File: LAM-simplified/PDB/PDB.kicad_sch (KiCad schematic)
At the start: 22 parts, among them J1 Conn_02x03_Counter_Clockwise, J10 Conn_01x02, J11 Conn_01x02, J12 Conn_01x02, J13 Conn_01x02, J14 Conn_01x02, J15 Conn_01x02, J16 Conn_01x02, J2 Conn_02x03_Counter_Clockwise, J3 Conn_02x03_Counter_Clockwise, J4 Conn_02x03_Counter_Clockwise, J5 Conn_01x02, J6 Conn_01x02, J7 Conn_01x02, J8 Conn_01x02, J9 Conn_01x02

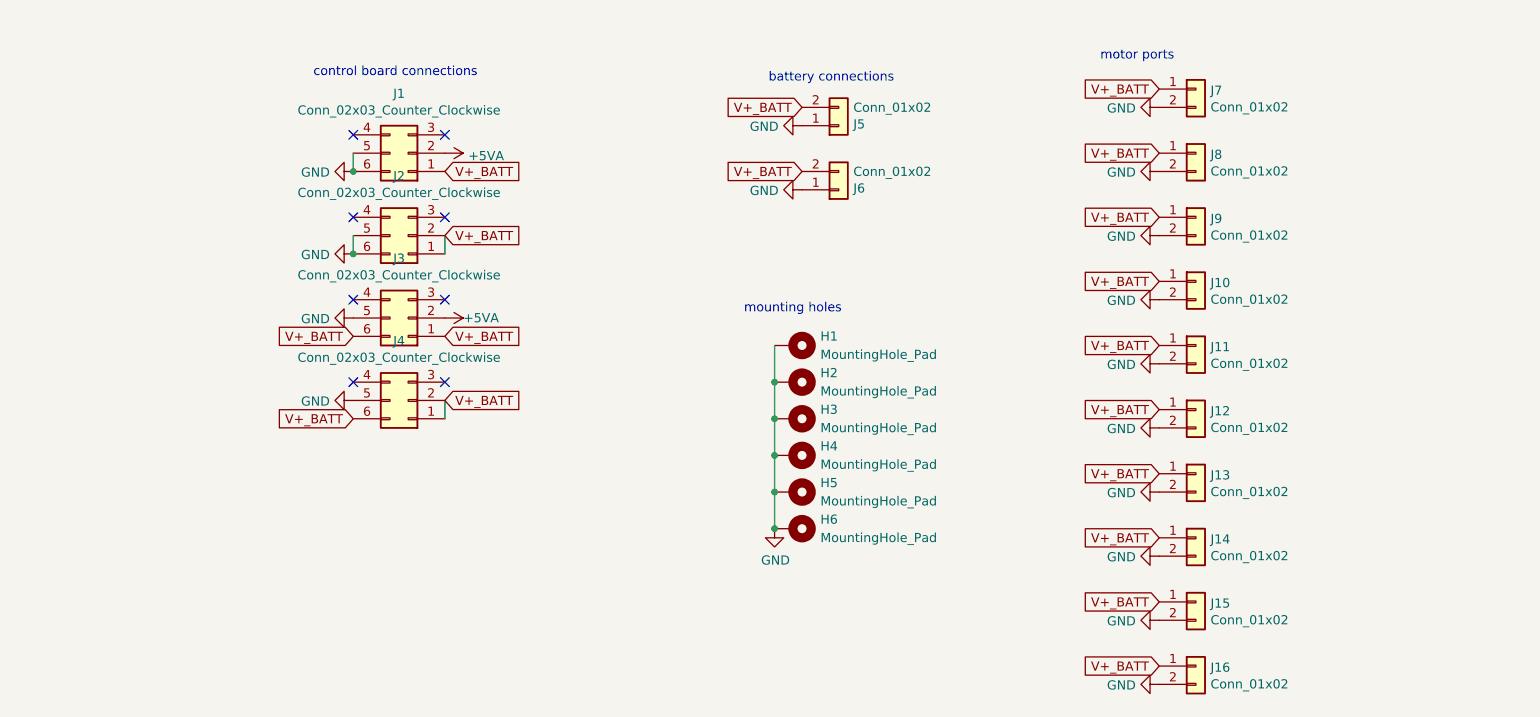
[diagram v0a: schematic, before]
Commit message: update LAM PDB PCB r1.3
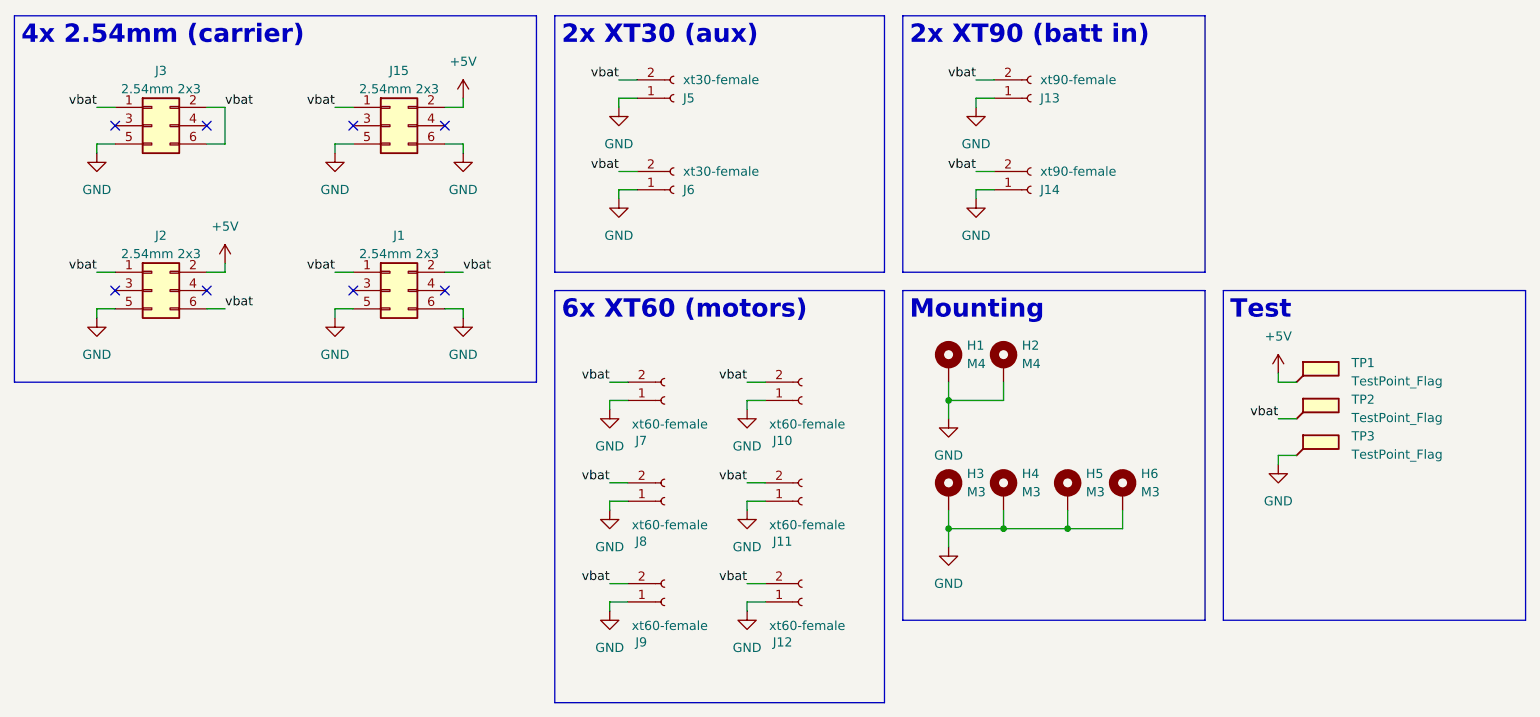
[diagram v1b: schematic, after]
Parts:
- removed J1, J2, J3, J4: Conn_02x03_Counter_Clockwise, Connector_PinHeader_2.54mm:PinHeader_2x03_P2.54mm_Vertical, symbol Connector_Generic:Conn_02x03_Counter_Clockwise
- removed J10, J11, J12, J13, J14, J15, J16, J7, J8, J9: Conn_01x02, PDB:XT-60_horizontal, symbol Connector_Generic:Conn_01x02
- removed J5, J6: Conn_01x02, Connector_AMASS:AMASS_XT30PW-F_1x02_P2.50mm_Horizontal, symbol Connector_Generic:Conn_01x02
- added J1, J15, J2, J3: 2.54mm 2x3, Connector_PinHeader_2.54mm:PinHeader_2x03_P2.54mm_Vertical, symbol Connector_Generic:Conn_02x03_Odd_Even
- added J10, J11, J12, J7, J8, J9: xt60-female, Connector_AMASS:AMASS_XT60PW-F_1x02_P7.20mm_Horizontal, symbol Connector:Conn_01x02_Socket
- added J13, J14: xt90-female, Connector_AMASS:AMASS_XT90PW-M_1x02_P10.90mm_Horizontal, symbol Connector:Conn_01x02_Socket
- added J5, J6: xt30-female, Connector_AMASS:AMASS_XT30PW-F_1x02_P2.50mm_Horizontal, symbol Connector:Conn_01x02_Socket
- added TP1, TP2, TP3: TestPoint_Flag, TestPoint:TestPoint_Keystone_5010-5014_Multipurpose, symbol Connector:TestPoint_Flag
- H1, H2: value MountingHole_Pad -> M4; footprint (none) -> TestPoint:TestPoint_Plated_Hole_D4.0mm; now left out of the parts list
- H3, H4, H5, H6: value MountingHole_Pad -> M3; footprint (none) -> MountingHole:MountingHole_3.2mm_M3_DIN965_Pad; now left out of the parts list
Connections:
- net GND: now also J1.5 (Pin_5), J1.6 (Pin_6), J10.1 (Pin_1), J11.1 (Pin_1), J12.1 (Pin_1), J13.1 (Pin_1), J14.1 (Pin_1), J15.5 (Pin_5), J15.6 (Pin_6), J2.5 (Pin_5), J3.5 (Pin_5), J5.1 (Pin_1), J6.1 (Pin_1), J7.1 (Pin_1), J8.1 (Pin_1), J9.1 (Pin_1), TP3.1
- new net +5V: J15.2 (Pin_2), J2.2 (Pin_2), TP1.1
- new net vbat: J1.1 (Pin_1), J1.2 (Pin_2), J10.2 (Pin_2), J11.2 (Pin_2), J12.2 (Pin_2), J13.2 (Pin_2), J14.2 (Pin_2), J15.1 (Pin_1), J2.1 (Pin_1), J2.6 (Pin_6), J3.1 (Pin_1), J3.2 (Pin_2), J3.6 (Pin_6), J5.2 (Pin_2), J6.2 (Pin_2), J7.2 (Pin_2), J8.2 (Pin_2), J9.2 (Pin_2), TP2.1
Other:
- note removed: "battery connections"
- note removed: "control board connections"
- note removed: "motor ports"
- note removed: "mounting holes"

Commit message: add BOM
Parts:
- J10, J11, J12, J7, J8, J9: lcsc (none) -> C428722
- J13, J14: lcsc (none) -> C3040690
- J5, J6: lcsc (none) -> C2913282
- TP1, TP2, TP3: lcsc (none) -> C2906765
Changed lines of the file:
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@@
+			)
+		)
+		(property "lcsc" "C2913282"
+			(at 107.95 26.67 0)
+			(effects
+				(font
+					(size 1.27 1.27)
+				)
+				(hide yes)
 			)
 		)
@@
 			)
 		)
+		(property "lcsc" ""
+			(at 68.58 30.48 0)
+			(effects
+				(font
+					(size 1.27 1.27)
+				)
+				(hide yes)
+			)
+		)
 		(pin "1"
 		)
@@
 			)
 		)
+		(property "lcsc" ""
+			(at 68.58 53.34 0)
+			(effects
+				(font
+					(size 1.27 1.27)
+				)
+				(hide yes)
+			)
+		)
 		(pin "1"
 		)
@@
 			)
 		)
+		(property "lcsc" ""
+			(at 35.56 30.48 0)
+			(effects
+				(font
+					(size 1.27 1.27)
+				)
+				(hide yes)
+			)
+		)
 		(pin "1"
 		)
@@
 			)
 		)
+		(property "lcsc" "C2913282"
+			(at 107.95 39.37 0)
+			(effects
+				(font
+					(size 1.27 1.27)
+				)
+				(hide yes)
+			)
+		)
 		(pin "1"
 		)
@@
 			)
 		)
+		(property "lcsc" "C428722"
+			(at 106.68 68.58 0)
+			(effects
+				(font
+					(size 1.27 1.27)
+				)
+				(hide yes)
+			)
+		)
 		(pin "2"
 		)
@@
 			)
 		)
+		(property "lcsc" "C428722"
+			(at 125.73 68.58 0)
+			(effects
+				(font
+					(size 1.27 1.27)
+				)
+				(hide yes)
+			)
+		)
 		(pin "2"
 		)
@@
 			)
 		)
+		(property "lcsc" "C2906765"
+			(at 194.31 71.12 0)
+			(effects
+				(font
+					(size 1.27 1.27)
+				)
+				(hide yes)
+			)
+		)
 		(pin "1"
 		)
@@
 			)
 		)
+		(property "lcsc" "C428722"
+			(at 106.68 96.52 0)
+			(effects
+				(font
+					(size 1.27 1.27)
+				)
+				(hide yes)
+			)
+		)
 		(pin "2"
 		)
@@
 			)
 		)
+		(property "lcsc" ""
+			(at 146.05 81.28 0)
+			(effects
+				(font
+					(size 1.27 1.27)
+				)
+				(hide yes)
+			)
+		)
 		(pin "1"
 		)
@@
 			)
 		)
+		(property "lcsc" "C428722"
+			(at 106.68 82.55 0)
+			(effects
+				(font
+					(size 1.27 1.27)
+				)
+				(hide yes)
+			)
+		)
 		(pin "2"
 		)
@@
 		)
 		(property "Description" "Mounting Hole with connection"
+			(at 170.18 81.28 0)
+			(effects
+				(font
+					(size 1.27 1.27)
+				)
+				(hide yes)
+			)
+		)
+		(property "lcsc" ""
 			(at 170.18 81.28 0)
 			(effects
@@
 			)
 		)
+		(property "lcsc" ""
+			(at 153.67 81.28 0)
+			(effects
+				(font
+					(size 1.27 1.27)
+				)
+				(hide yes)
+			)
+		)
 		(pin "1"
 		)
@@
 			)
 		)
+		(property "lcsc" "C2906765"
+			(at 194.31 66.04 0)
+			(effects
+				(font
+					(size 1.27 1.27)
+				)
+				(hide yes)
+			)
+		)
 		(pin "1"
 		)
@@
 		)
 		(property "Description" "Mounting Hole with connection"
+			(at 162.56 81.28 0)
+			(effects
+				(font
+					(size 1.27 1.27)
+				)
+				(hide yes)
+			)
+		)
+		(property "lcsc" ""
 			(at 162.56 81.28 0)
 			(effects
@@
 			)
 		)
+		(property "lcsc" "C3040690"
+			(at 157.48 26.67 0)
+			(effects
+				(font
+					(size 1.27 1.27)
+				)
+				(hide yes)
+			)
+		)
 		(pin "2"
 		)
@@
 		)
 		(property "Description" "Mounting Hole with connection"
+			(at 153.67 63.5 0)
+			(effects
+				(font
+					(size 1.27 1.27)
+				)
+				(hide yes)
+			)
+		)
+		(property "lcsc" ""
 			(at 153.67 63.5 0)
 			(effects
@@
 			)
 		)
+		(property "lcsc" "C428722"
+			(at 125.73 82.55 0)
+			(effects
+				(font
+					(size 1.27 1.27)
+				)
+				(hide yes)
+			)
+		)
 		(pin "2"
 		)
@@
 		)
 		(property "Description" "Mounting Hole with connection"
+			(at 146.05 63.5 0)
+			(effects
+				(font
+					(size 1.27 1.27)
+				)
+				(hide yes)
+			)
+		)
+		(property "lcsc" ""
 			(at 146.05 63.5 0)
 			(effects
@@
 			)
 		)
+		(property "lcsc" "C428722"
+			(at 125.73 96.52 0)
+			(effects
+				(font
+					(size 1.27 1.27)
+				)
+				(hide yes)
+			)
+		)
 		(pin "2"
 		)
@@
 			)
 		)
+		(property "lcsc" "C2906765"
+			(at 194.31 76.2 0)
+			(effects
+				(font
+					(size 1.27 1.27)
+				)
+				(hide yes)
+			)
+		)
 		(pin "1"
 		)
@@
 			)
 		)
+		(property "lcsc" "C3040690"
+			(at 157.48 39.37 0)
+			(effects
+				(font
+					(size 1.27 1.27)
+				)
+				(hide yes)
+			)
+		)
 		(pin "2"
 		)
@@
 			(at 35.56 53.34 0)
 			(effects
+				(font
+					(size 1.27 1.27)
+				)
+				(hide yes)
+			)
+		)
+		(property "lcsc" ""
+			(at 35.56 53.34 0)
+			(effects
